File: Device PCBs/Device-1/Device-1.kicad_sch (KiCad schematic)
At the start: 31 parts, among them J1 Conn_01x04_Female, J2 Conn_01x04_Female, U1 EBYTE_E32-433T20D, U2 MAX487E

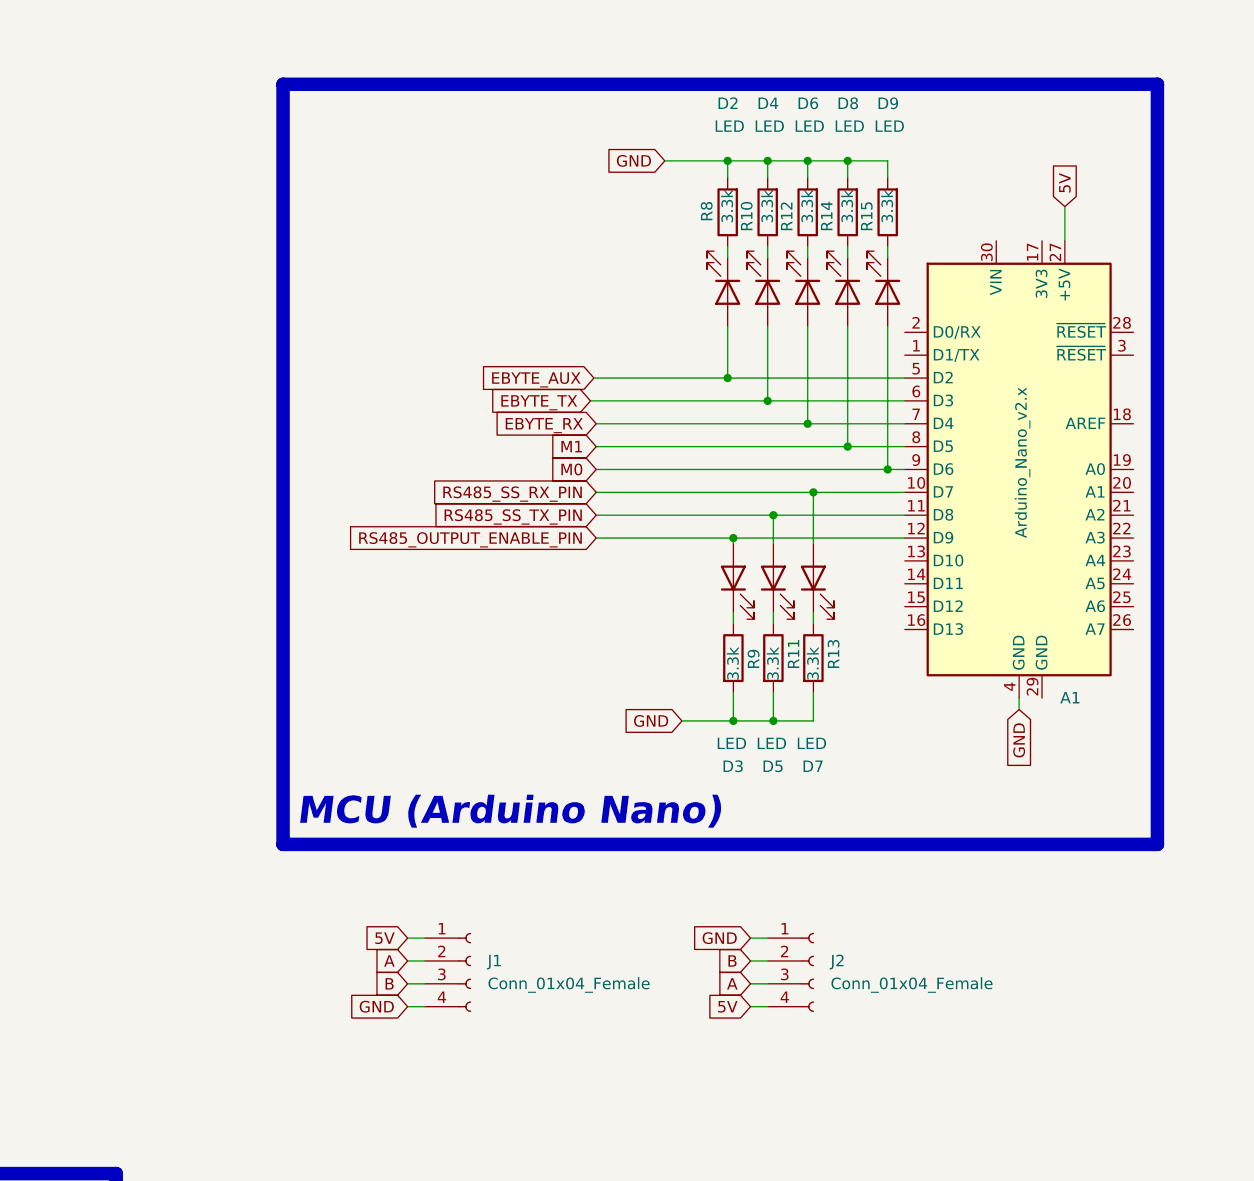
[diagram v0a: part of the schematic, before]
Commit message: Device 1 PCB is finished
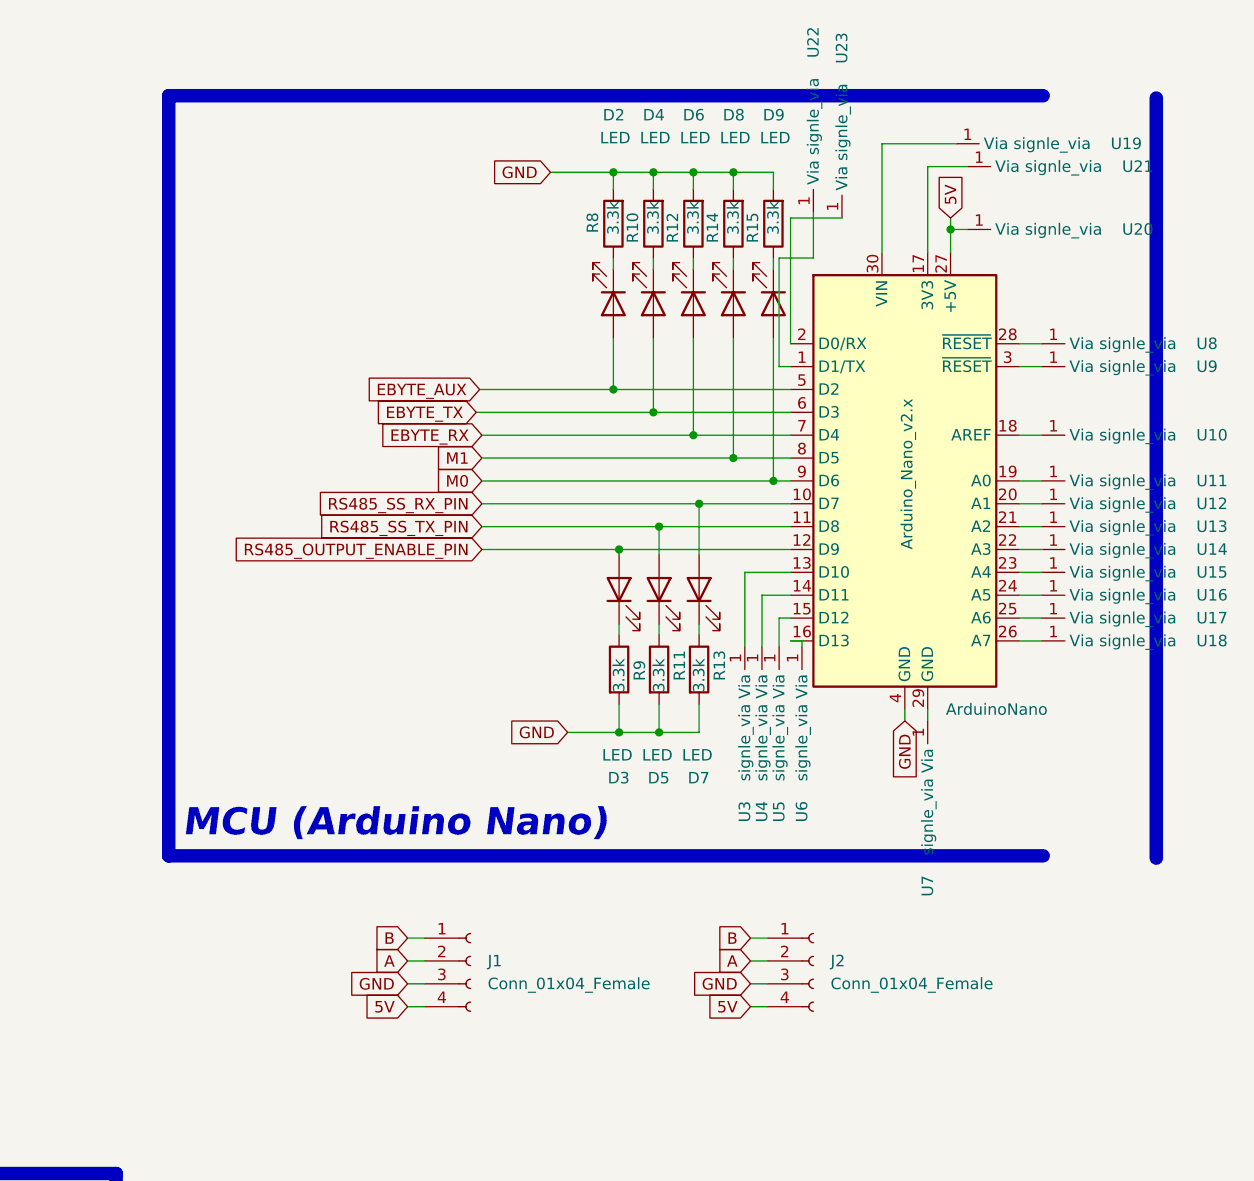
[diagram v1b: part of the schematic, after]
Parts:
- added U10, U11, U12, U13, U14, U15, U16, U17, U18, U19, U20, U21, U22, U23, U3, U4, U5, U6, U7, U8, U9: signle_via, Device_1_project_footprints:single_via, symbol device_1_project_symbols:signle_via
- C1: footprint Capacitor_SMD:CP_Elec_6.3x5.7 -> Capacitor_SMD:CP_Elec_6.3x5.2
- D1, D2, D3, D8, D9: footprint LED_SMD:LED_1206_3216Metric -> Device_1_project_footprints:lm281B-3000K
- D4, D5, D6, D7: footprint LED_SMD:LED_1206_3216Metric -> Device_1_project_footprints:lm281B-6500K
- renumbered A1 to ArduinoNano
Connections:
- net 5V: now also J1.4 (Pin_4), U20.1 (Via); no longer J1.1 (Pin_1)
- net A: now also J2.2 (Pin_2); no longer J2.3 (Pin_3)
- net B: now also J1.1 (Pin_1), J2.1 (Pin_1); no longer J1.3 (Pin_3), J2.2 (Pin_2)
- net GND: now also J1.3 (Pin_3), J2.3 (Pin_3); no longer J1.4 (Pin_4), J2.1 (Pin_1)
- net at ArduinoNano.1 (D1/TX): now also U22.1 (Via)
- net at ArduinoNano.13 (D10): now also U3.1 (Via)
- net at ArduinoNano.14 (D11): now also U4.1 (Via)
- net at ArduinoNano.15 (D12): now also U5.1 (Via)
- net at ArduinoNano.16 (D13): now also U6.1 (Via)
- net at ArduinoNano.17 (3V3): now also U21.1 (Via)
- net at ArduinoNano.18 (AREF): now also U10.1 (Via)
- net at ArduinoNano.19 (A0): now also U11.1 (Via)
- net at ArduinoNano.2 (D0/RX): now also U23.1 (Via)
- net at ArduinoNano.20 (A1): now also U12.1 (Via)
- net at ArduinoNano.21 (A2): now also U13.1 (Via)
- net at ArduinoNano.22 (A3): now also U14.1 (Via)
- net at ArduinoNano.23 (A4): now also U15.1 (Via)
- net at ArduinoNano.24 (A5): now also U16.1 (Via)
- net at ArduinoNano.25 (A6): now also U17.1 (Via)
- net at ArduinoNano.26 (A7): now also U18.1 (Via)
- net at ArduinoNano.28 (~{RESET}): now also U8.1 (Via)
- net at ArduinoNano.29 (GND): now also U7.1 (Via)
- net at ArduinoNano.3 (~{RESET}): now also U9.1 (Via)
- net at ArduinoNano.30 (VIN): now also U19.1 (Via)
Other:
- moved on the sheet: ArduinoNano, D2, D3, D4, D5, D6, D7, D8, D9, R10, R11, R12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
